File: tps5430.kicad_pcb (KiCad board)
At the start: 2 copper layers, 17.5 x 22 mm, 12 parts, among them J1 Conn_01x01_Pin, J2 Conn_01x01_Pin, J3 Conn_01x01_Pin, J4 Conn_01x01_Pin, U1 TPS5430DDA

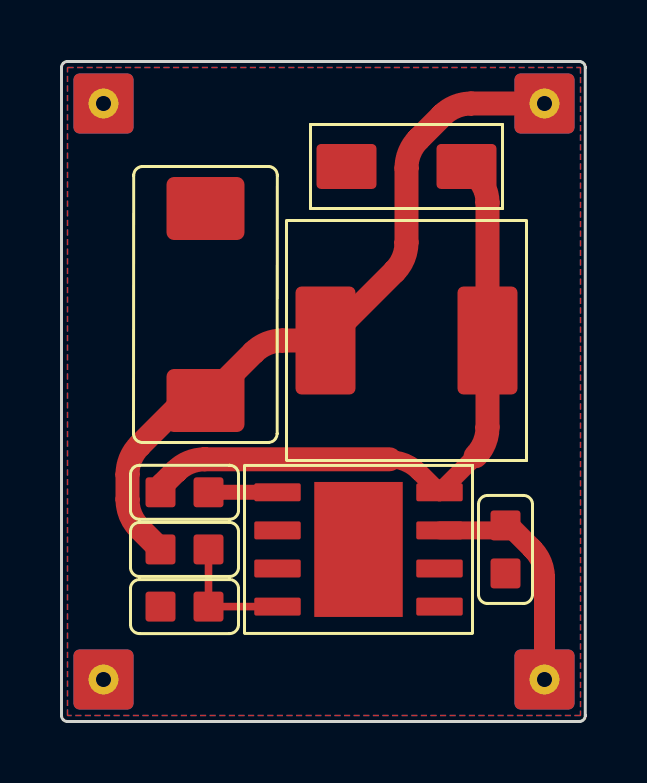
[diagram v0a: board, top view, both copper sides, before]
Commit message: done
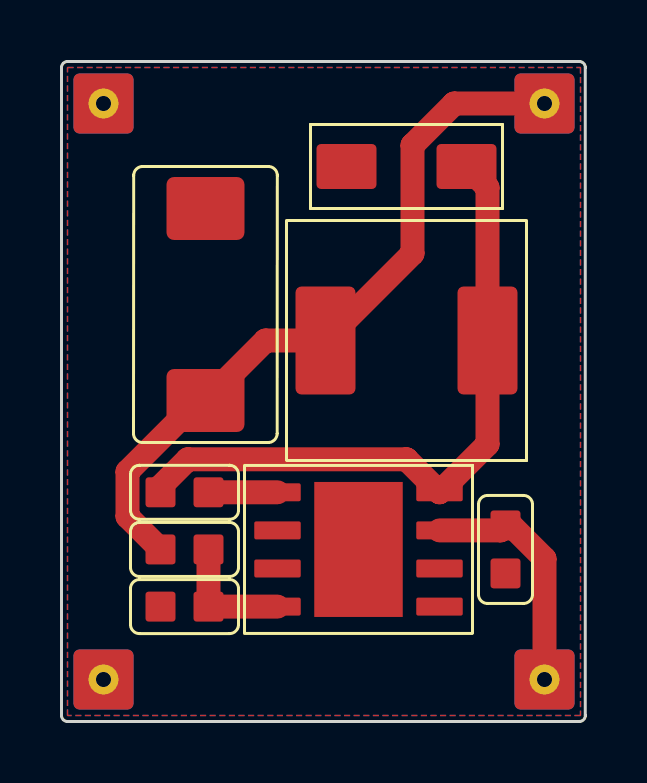
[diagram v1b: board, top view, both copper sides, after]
